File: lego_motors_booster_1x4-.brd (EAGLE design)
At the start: 40.6 x 65.4 mm, 21 parts, among them Q1 IRF4905, Q3 BS170T, Q5 BUZ11BV, X1 NXT-SOCKET, X2 NXT-SOCKET, X3 NXT-SOCKET, X4 NXT-SOCKET, X5 NXT-SOCKET

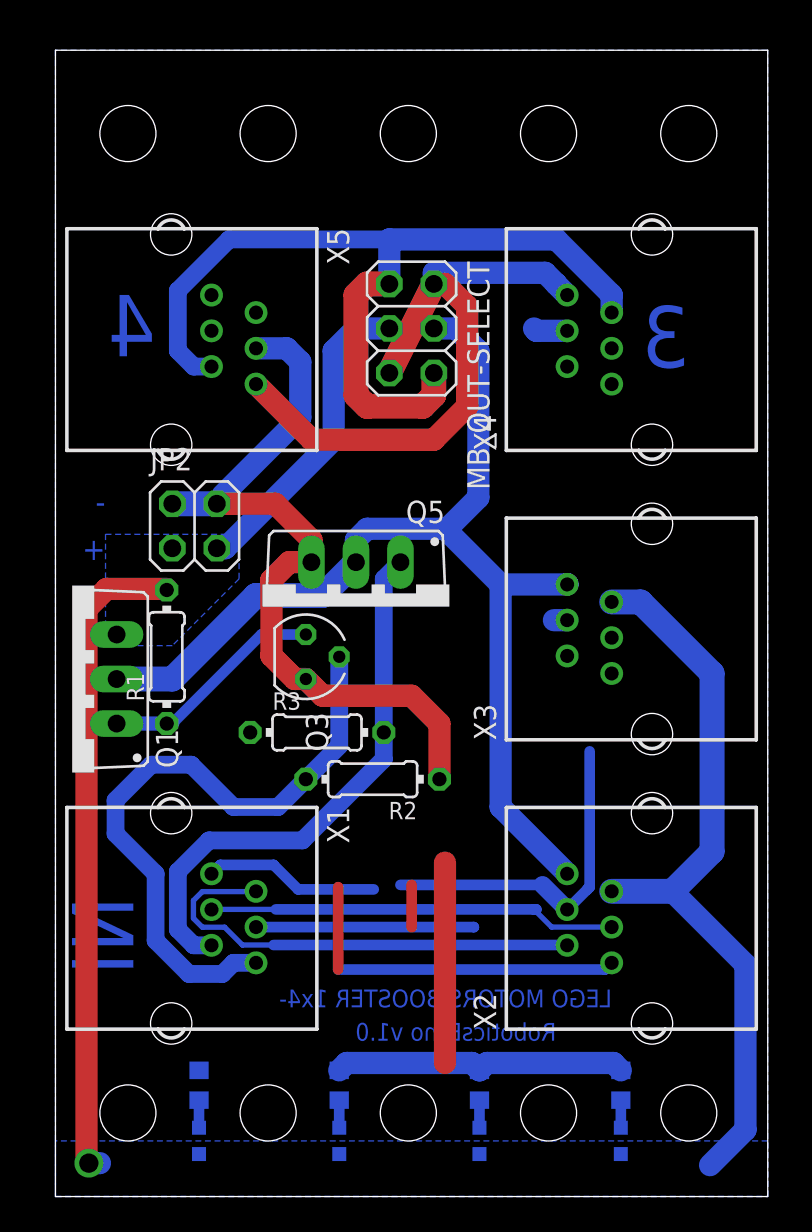
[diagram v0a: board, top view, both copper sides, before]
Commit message: mirrored + maybe some minor improvements
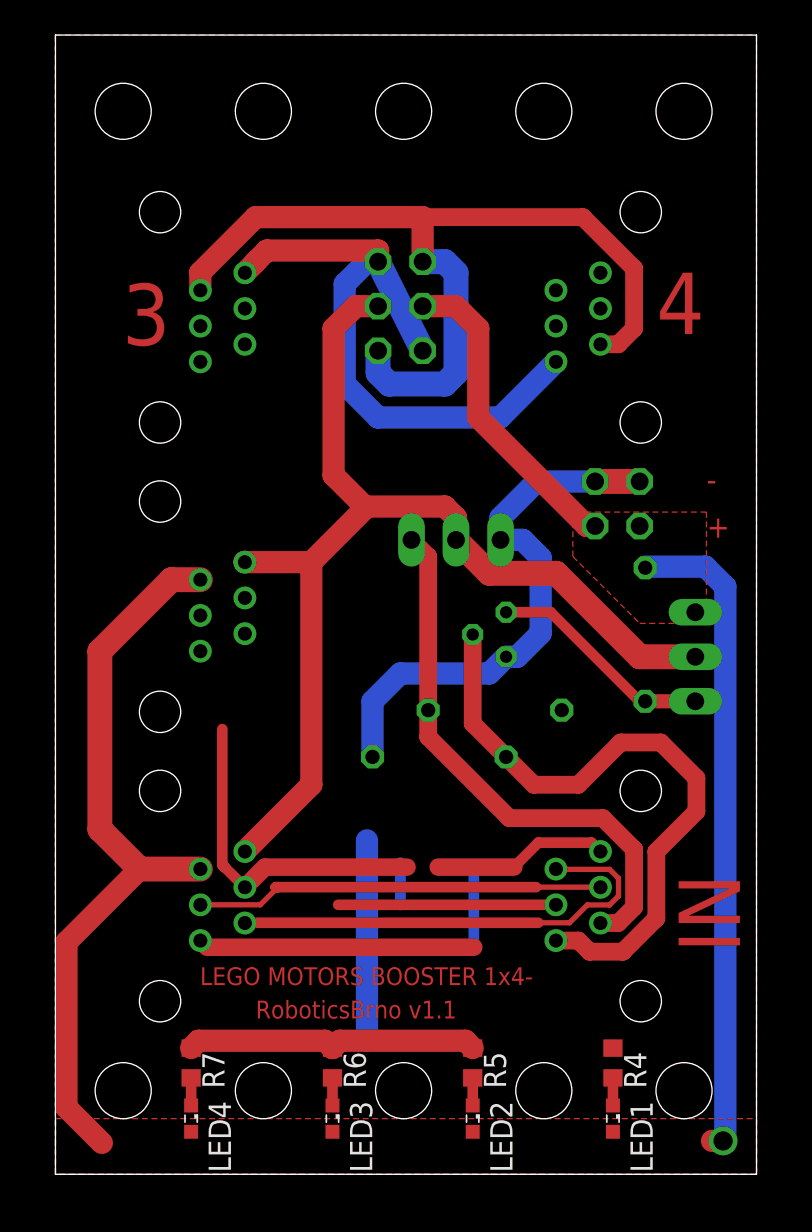
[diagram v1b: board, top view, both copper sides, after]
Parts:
- moved X2 40.0 mm to (0.00, 15.9), flipped to the bottom
- moved X3 40.0 mm to (0.00, 32.4), flipped to the bottom
- moved X4 40.0 mm to (0.00, 48.9), flipped to the bottom
- moved X1 38.8 mm to (39.4, 15.9), flipped to the bottom
- moved X5 38.8 mm to (39.4, 48.9), flipped to the bottom
- moved Q1 38.1 mm to (39.0, 29.5), flipped to the bottom
- moved R1 27.3 mm to (33.6, 30.8), flipped to the bottom
- moved LED4 24.5 mm to (7.74, 3.17), flipped to the top
- moved R7 24.5 mm to (7.74, 6.35), flipped to the top
- moved JP2 24.2 mm to (32.1, 38.3), flipped to the bottom
- moved LED1 23.7 mm to (31.8, 3.17), flipped to the top
- moved R4 23.7 mm to (31.8, 6.35), flipped to the top
- moved Q3 11.5 mm to (25.7, 30.8), flipped to the bottom
- moved R3 10.2 mm to (25.1, 26.5), flipped to the bottom
- moved LED3 8.48 mm to (15.8, 3.17), flipped to the top
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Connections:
- removed net N$11: X4.4
- removed net N$12: X4.5
- removed net N$13: X4.6
- removed net N$17: X5.4
- removed net N$18: X5.5
- removed net N$19: X5.6
- removed net N$5: X3.4
- removed net N$6: X3.5
- removed net N$7: X3.6
- net GND: no longer X3.3, X4.3, X5.3
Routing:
- net GND: track 106.7 -> 91.4 mm
- added copper zone on layer 1, net GND
- added copper zone on layer 1, net VCC
- removed copper zone on layer 16, net GND
- removed copper zone on layer 16, net VCC
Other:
- board size 40.6 x 65.4 mm -> 40 x 65 mm
- board text added: "RoboticsBrno v1.1"
- board text removed: "RoboticsBrno v1.0"
